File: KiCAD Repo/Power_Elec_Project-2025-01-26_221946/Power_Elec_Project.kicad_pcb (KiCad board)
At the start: 2 copper layers, 40 parts, among them U2 LAUNCHXL-F28379D, U3 UCC5304DWVR, U4 TMV 0512SHI, U5 AMC1300DWVR

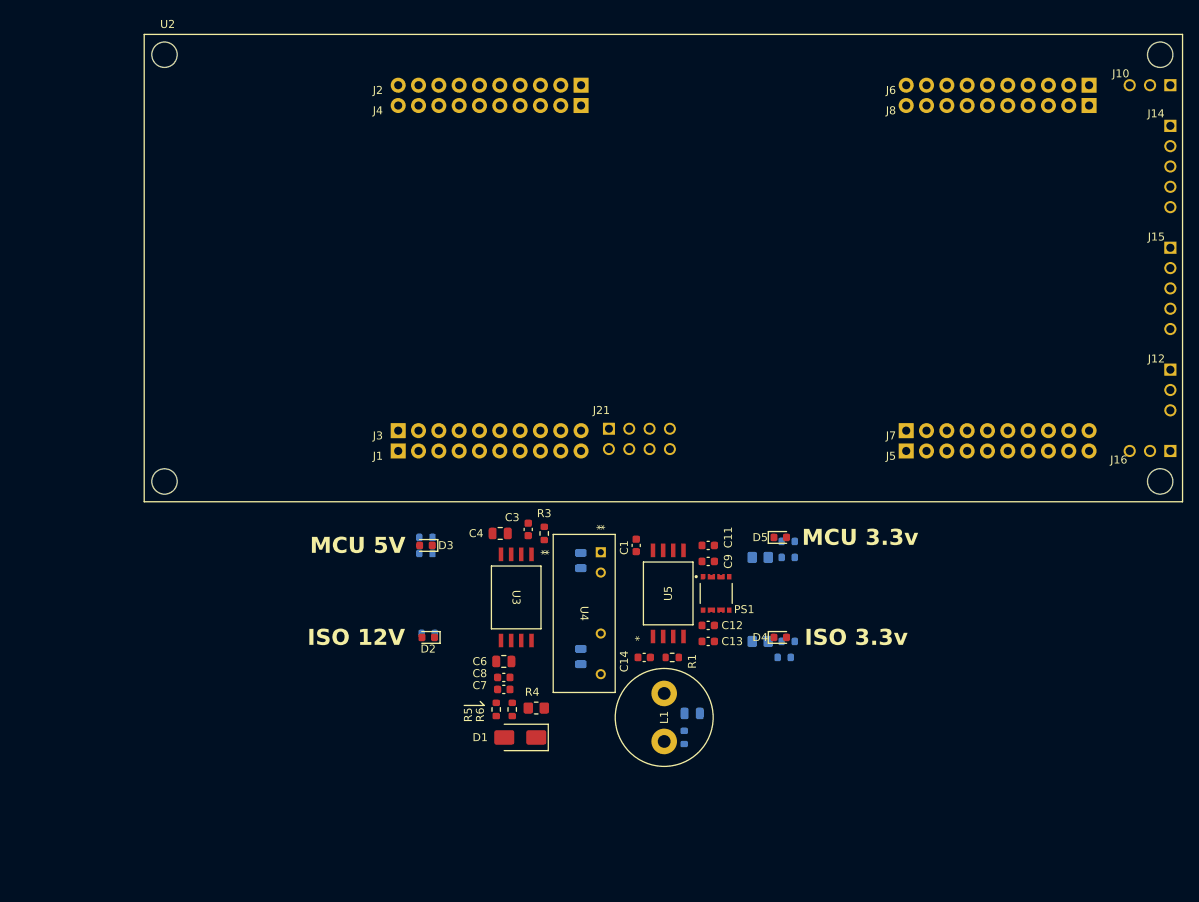
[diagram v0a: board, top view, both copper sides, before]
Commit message: PCB layout
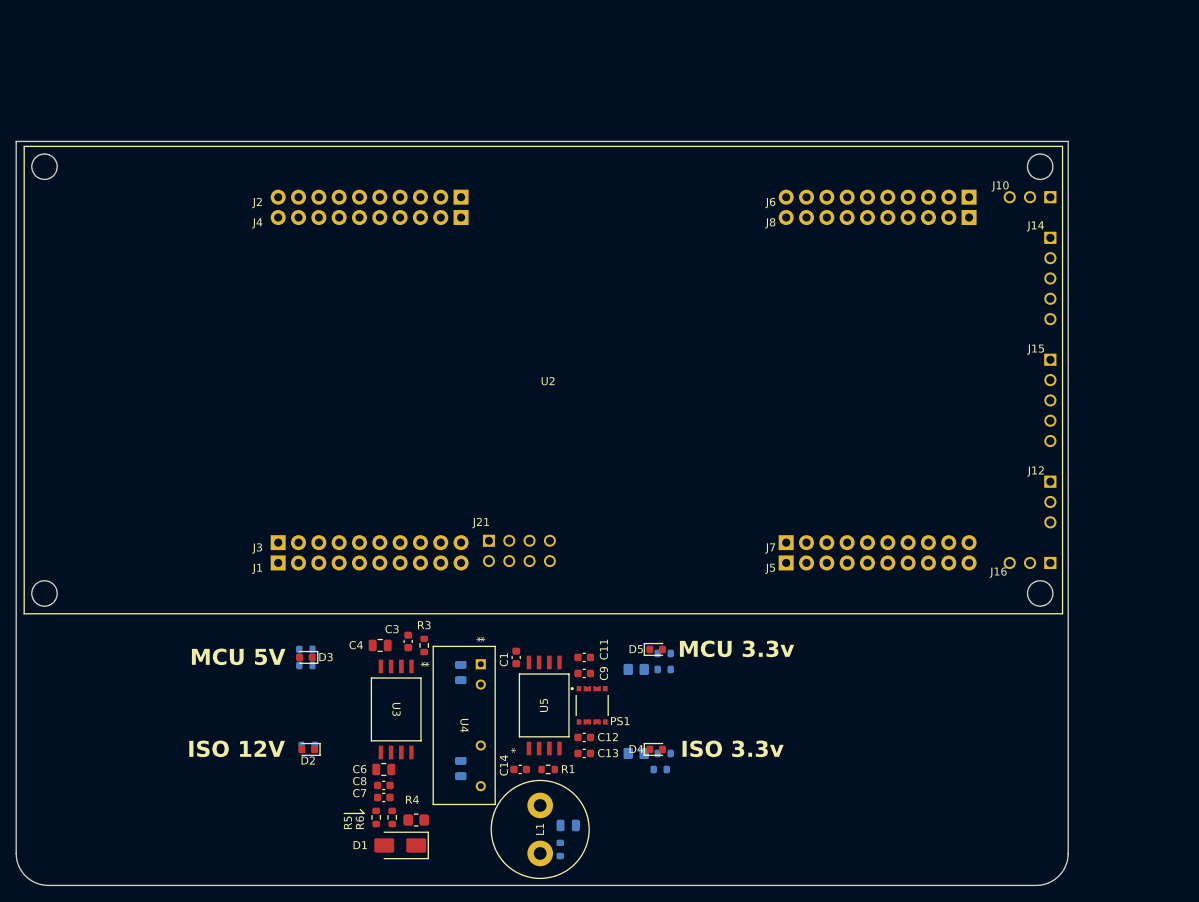
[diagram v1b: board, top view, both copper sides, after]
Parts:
- moved C11 20.9 mm to (110.5, 122.0)
- moved C12 20.9 mm to (110.5, 132.0)
- moved C13 20.9 mm to (110.5, 134.0)
- moved C14 20.9 mm to (102.5, 136.0)
- moved C2 20.9 mm to (108.5, 143.0)
- moved C9 20.9 mm to (110.5, 124.0)
- moved D4 20.9 mm to (119.5, 133.5)
- moved D5 20.9 mm to (119.5, 121.0)
- moved L1 20.9 mm to (105.0, 146.5)
- moved PS1 20.9 mm to (111.5, 128.0)
- moved R1 20.9 mm to (106.0, 136.0)
- moved R10 20.9 mm to (120.5, 134.0)
- moved R11 20.9 mm to (120.0, 136.0)
- moved R12 20.9 mm to (117.0, 134.0)
- moved R13 20.9 mm to (117.0, 123.5)
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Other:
- board outline added: 131.5 x 93 mm
